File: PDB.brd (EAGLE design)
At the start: 125.9 x 103 mm, 50 parts, among them J1 B06B-HCMKK, J2 B06B-HCMKK, J3 SS-6488-NF-A431, J4 SS-6488-NF-A431, J5 B06B-HCMKK, J6 B03B-HCMKS, J7 B03B-HCMKS, J8 SS-6488-NF-A431

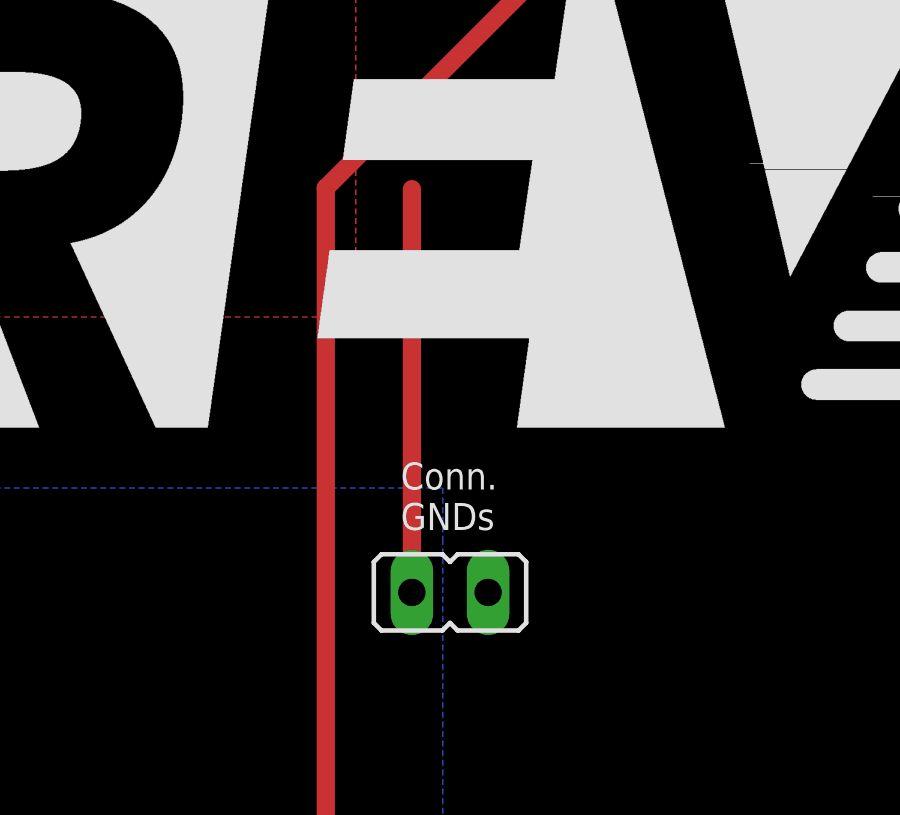
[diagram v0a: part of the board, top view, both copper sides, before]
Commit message: Schematic first version
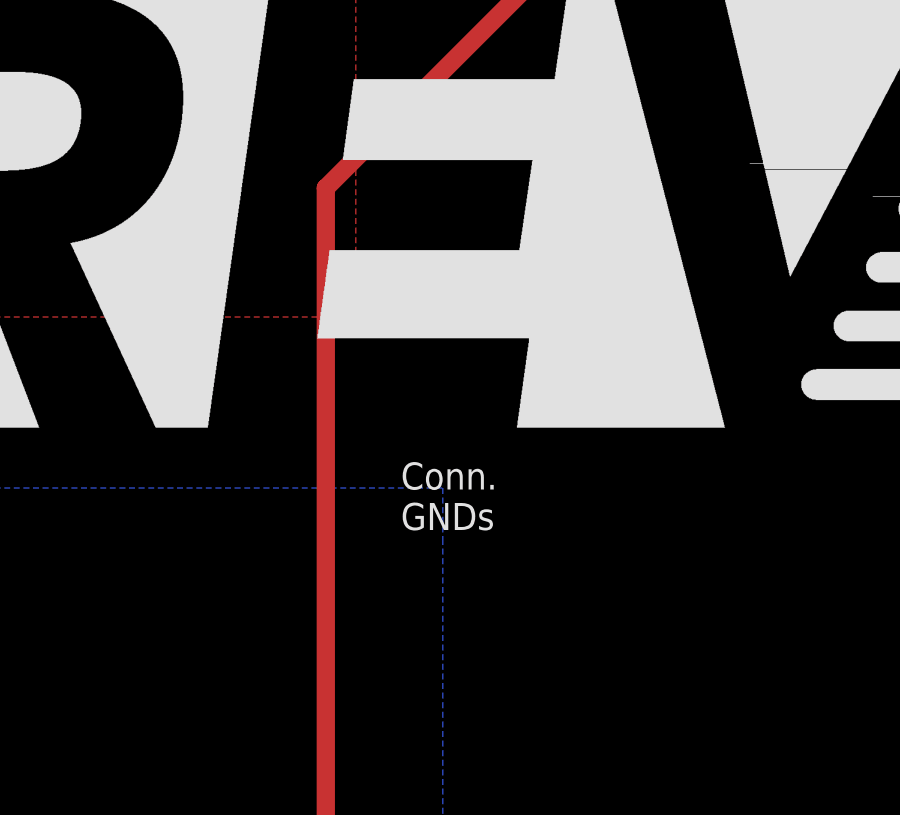
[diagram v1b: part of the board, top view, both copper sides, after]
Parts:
- removed JP1: (no value), jumper:JP1
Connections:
- removed net µC_GND: JP1.2
- new net VIPER: J2.3
- net GND: no longer JP1.1
- net HORN: now also J2.4
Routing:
- net µC_GND: track 13.4 -> 0.00 mm
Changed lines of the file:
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@@
 <element name="TRACO" library="master_library" package="SIP3" value="TRACO-TSR-1-2450" x="120.78" y="101.56" smashed="yes"/>
 <element name="LM2940" library="master_library" package="SOT230P700X180-4" package3d_urn="urn:adsk.eagle:package:8814566/1" value="LM2940LM" x="30.48" y="112.8" smashed="yes"/>
-<element name="JP1" library="jumper" library_urn="urn:adsk.eagle:library:252" package="JP1" package3d_urn="urn:adsk.eagle:package:15455/1" value="" x="105.14" y="66.52" smashed="yes" rot="R90">
-<attribute name="POPULARITY" value="15" x="105.14" y="66.52" size="1.778" layer="27" rot="R90" display="off"/>
-<attribute name="VALUE" x="107.68" y="69.441" size="1.27" layer="27" ratio="10" rot="R180"/>
-</element>
 <element name="C5" library="SparkFun-Capacitors" library_urn="urn:adsk.eagle:library:510" package="PANASONIC_C" package3d_urn="urn:adsk.eagle:package:37430/1" value="47uF" x="22.2" y="112.9" smashed="yes" rot="R270">
 <attribute name="NAME" x="24.867" y="112.9" size="0.6096" layer="25" font="vector" ratio="20" rot="R270" align="bottom-center"/>
@@
 </signal>
 <signal name="µC_GND">
-<contactref element="JP1" pad="2"/>
 <polygon width="0.2" layer="16" isolate="0.254">
 <vertex x="104.9" y="68.3"/>
@@
 <vertex x="104.9" y="70"/>
 </polygon>
-<wire x1="103.87" y1="66.52" x2="103.87" y2="79.962" width="0.6096" layer="1"/>
 </signal>
 <signal name="5V_REG">
@@
 <wire x1="106.34" y1="108.42" x2="103.6645" y2="108.42" width="0.6096" layer="1"/>
 <wire x1="103.435" y1="108.312" x2="103.6645" y2="108.42" width="0.6096" layer="1"/>
-<contactref element="JP1" pad="1"/>
 <contactref element="R5" pad="2"/>
 <contactref element="HAZ_R" pad="2"/>
@@
 <wire x1="16.36" y1="88.56" x2="27.4532" y2="112.8" width="0" layer="19" extent="1-1"/>
 <wire x1="-13.92" y1="89.82" x2="15.72" y2="86.28" width="0" layer="19" extent="1-1"/>
-<wire x1="106.41" y1="66.52" x2="121.35" y2="97.6" width="0" layer="19" extent="1-1"/>
 <wire x1="1.32" y1="54.26" x2="15.72" y2="86.28" width="0" layer="19" extent="1-1"/>
 <wire x1="2.3" y1="20" x2="1.32" y2="54.26" width="0" layer="19" extent="1-1"/>
@@
 <wire x1="-43.83" y1="18.84" x2="-26.73" y2="18.84" width="0" layer="19" extent="1-1"/>
 <wire x1="-31.9" y1="-8.2" x2="-26.73" y2="18.84" width="0" layer="19" extent="1-1"/>
-<wire x1="66.48" y1="67.788" x2="106.41" y2="66.52" width="0" layer="19" extent="1-1"/>
+<wire x1="66.48" y1="67.788" x2="69.2" y2="109" width="0" layer="19" extent="1-1"/>
 <wire x1="-39.52" y1="-76.9" x2="-31.9" y2="-8.2" width="0" layer="19" extent="1-1"/>
 <wire x1="-47.82" y1="-91.11" x2="-39.52" y2="-76.9" width="0" layer="19" extent="1-1"/>
@@
 <signal name="HORN">
 <contactref element="U$5" pad="SWB"/>
+<contactref element="J2" pad="4"/>
+<wire x1="-2.78" y1="5.9" x2="-32.58" y2="-91.11" width="0" layer="19" extent="1-1"/>
 </signal>
 <signal name="MOSI_SW">
@@
 <wire x1="-13.92" y1="72.04" x2="-54.58" y2="-85.3" width="0" layer="19" extent="1-1"/>
 </signal>
+<signal name="VIPER">
+<contactref element="J2" pad="3"/>
+</signal>
 </signals>

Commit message: Board layout proposal
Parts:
- moved J8 207.7 mm to (112.5, 27.1), turned to 90 degrees
- moved U$6 198.5 mm to (27.0, 89.2), turned to 270 degrees
- moved U$5 194.8 mm to (42.8, 88.9), turned to 270 degrees
- moved HORN 174.8 mm to (72.3, 80.0)
- moved J2 161.9 mm to (78.0, 141.5)
- moved J5 150.4 mm to (92.1, 54.4), flipped to the bottom
- moved POWER1 145.3 mm to (58.6, 62.9)
- moved J1 135.2 mm to (48.3, 141.8)
- moved J6 134.1 mm to (22.4, 52.2), turned to 90 degrees
- moved R1 133.6 mm to (52.8, 62.8), turned to 180 degrees
- moved U$4 129.0 mm to (64.0, 54.6), turned to 90 degrees
- moved J4 127.6 mm to (82.2, 7.00)
- moved J7 123.9 mm to (22.7, 27.1), turned to 90 degrees
- moved U$2 111.0 mm to (44.8, 53.9), turned to 270 degrees
- moved J3 78.4 mm to (49.8, 6.50)
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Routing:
- net BRAKE_SNS: track 85.4 -> 17.8 mm, vias 1 -> 0
- net BRAKE_SIG: track 50.3 -> 0.00 mm
- net HAZ_L_SIG: track 46.5 -> 0.12 mm, vias 1 -> 0
- net 5V_REG: track 33.0 -> 3.99 mm
- net HAZ_R_SIG: track 33.9 -> 8.31 mm
- net H7: track 6.44 -> 32.0 mm
- net REARLIGHT_SIG: track 10.9 -> 0.00 mm
- net H4: track 8.35 -> 0.00 mm
- net HEADLIGHT_SIG: track 7.43 -> 0.00 mm
- net H3: track 6.53 -> 11.7 mm
- net H2: track 7.72 -> 11.1 mm
- net H8: track 6.54 -> 7.95 mm
- net CLK: track 0.82 -> 0.00 mm
- removed copper zone on layer 1, net 12V_IN
- removed copper zone on layer 16, net µC_GND
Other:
- board size 125.9 x 103 mm -> 126.8 x 162.5 mm
- board text removed: "12V IN"
- board text removed: "22uF"
- board text removed: "4.7k"
- board text removed: "555"
- board text removed: "ADD 1"
- board text removed: "Add 1"
- board text removed: "Add 2"
- board text removed: "BRAKE"
- board text removed: "Brake Light"
- board text removed: "Brake Sensor"
- board text removed: "Conn. GNDs"
- board text removed: "HL"
- board text removed: "Head Lights"
- board text removed: "ON"
- board text removed: "RL"
- board text removed: "Rear Lights"
- board text removed: "TURN_L"
- board text removed: "TURN_R"
- board text removed: "Wiper"
- board text removed: "µC"
- board text removed: "µC GND"

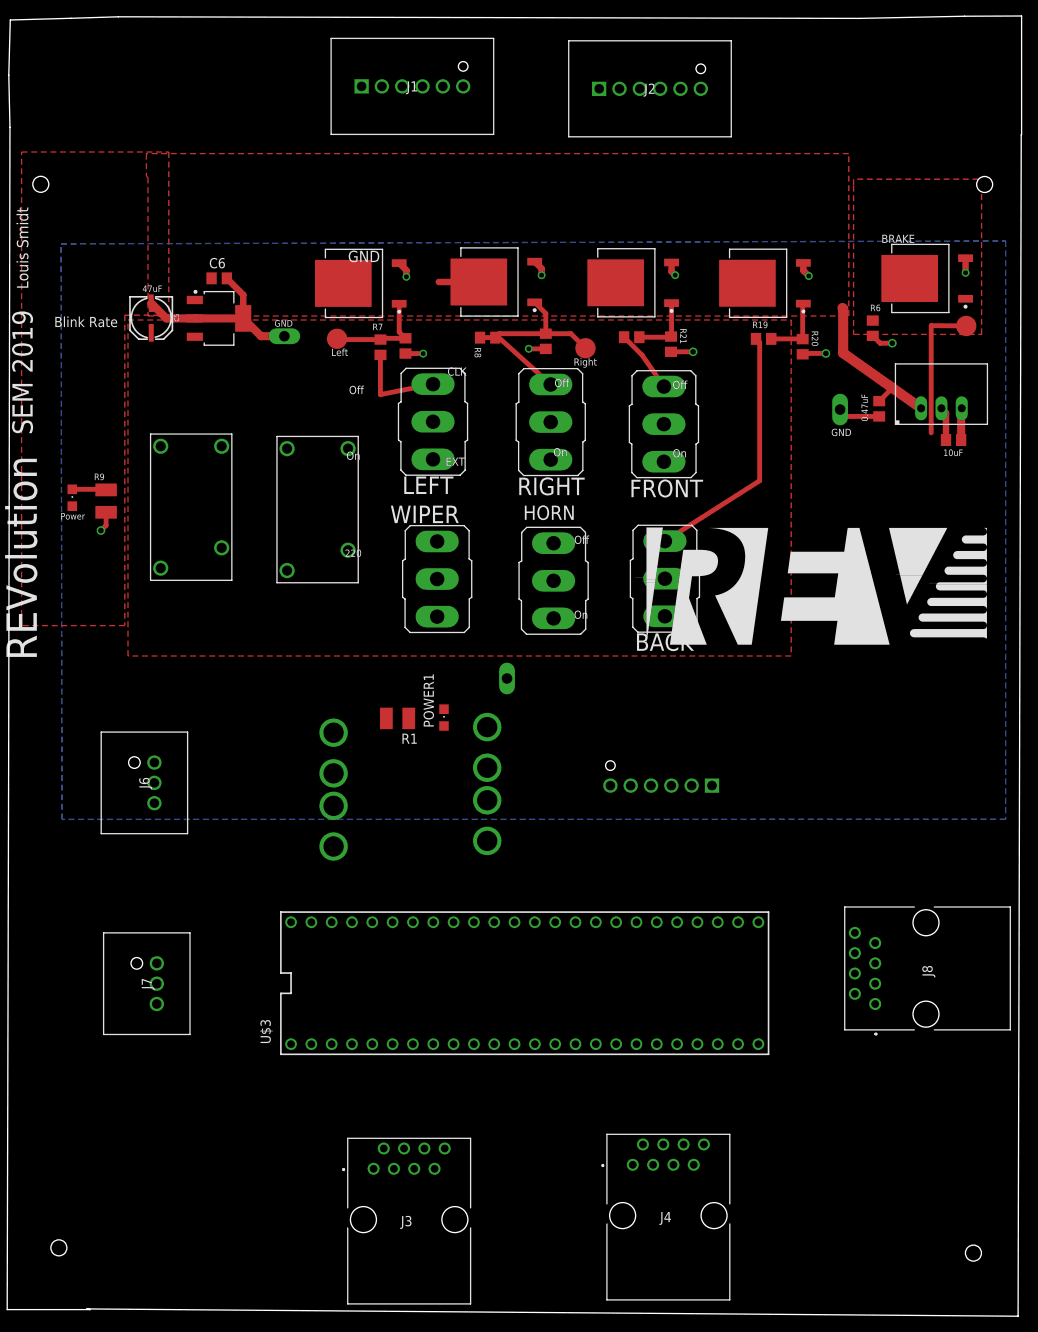
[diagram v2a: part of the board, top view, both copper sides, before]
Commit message: Board first version
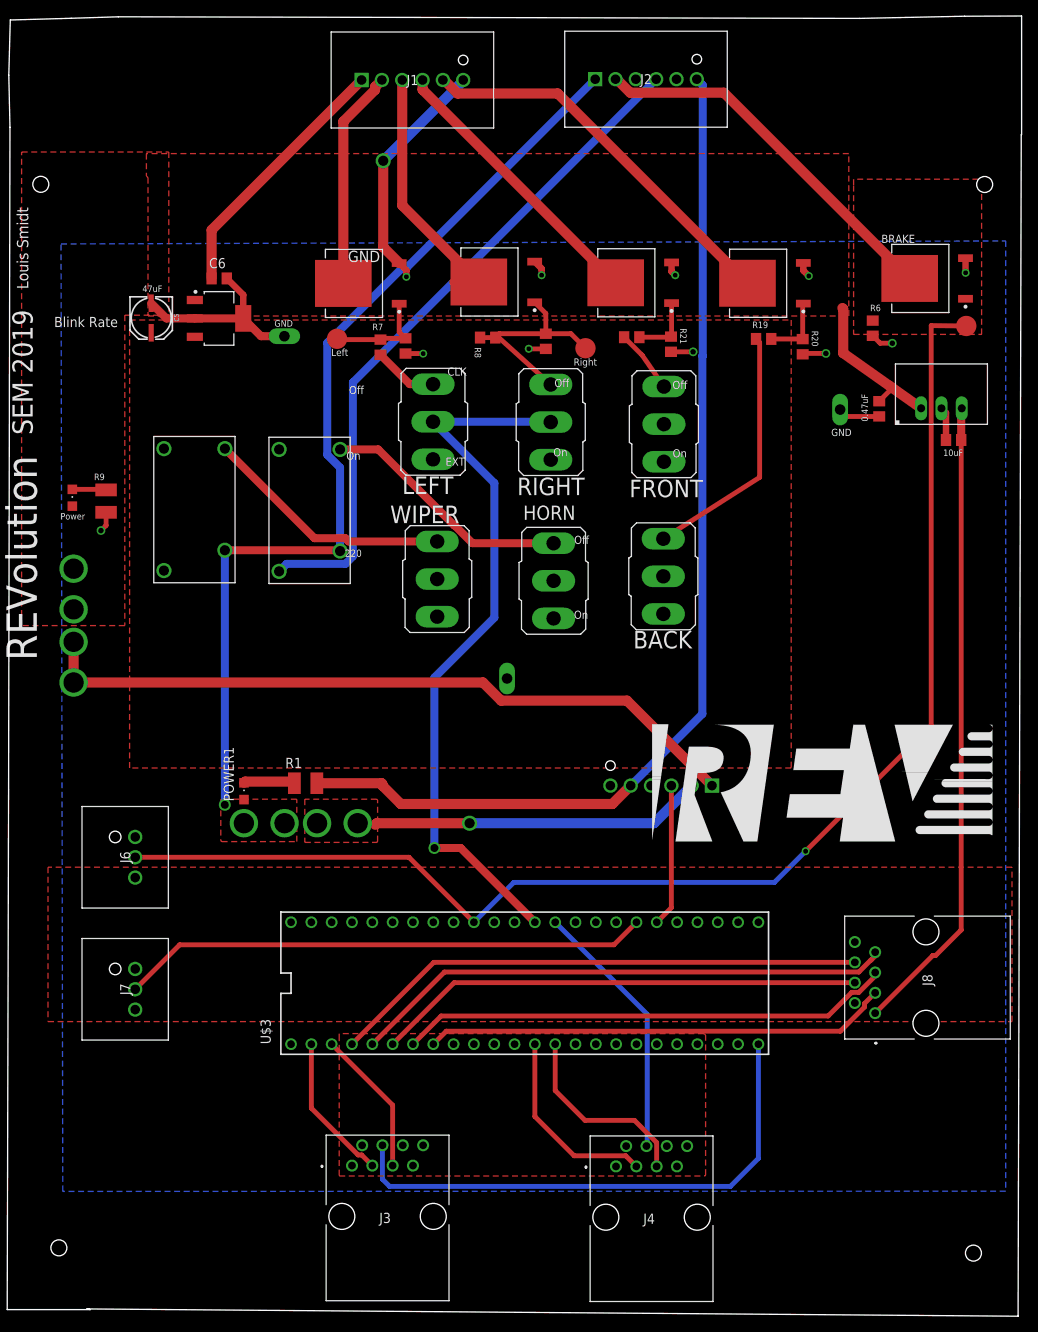
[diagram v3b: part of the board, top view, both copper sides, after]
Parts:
- moved U$2 38.4 mm to (12.3, 74.4)
- moved POWER1 26.6 mm to (33.6, 53.7)
- moved U$4 23.8 mm to (40.7, 49.7), turned to 180 degrees
- moved R1 14.1 mm to (41.3, 54.7), turned to 0 degrees
- moved J6 9.60 mm to (20.0, 42.9)
- moved J7 2.79 mm to (20.0, 26.4)
- moved J3 2.73 mm to (47.1, 6.90)
- moved J4 2.11 mm to (80.1, 6.80)
- moved J2 1.30 mm to (77.5, 142.7)
- moved J8 1.14 mm to (112.5, 26.0)
- moved U$5 1.00 mm to (41.8, 88.8)
- moved J1 0.80 mm to (48.3, 142.6)
- moved U$6 0.50 mm to (27.4, 88.9)
- moved BACK 0.36 mm to (86.0, 80.6)
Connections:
- removed net 5V: J7.1
- net 5V_REG: now also J7.1
- net CLK_SW: now also J8.6; no longer J8.4
- net CS: now also J8.4; no longer J8.6
- net MOSI_SW: now also J8.7; no longer J8.3
- net RESET: now also J8.3; no longer J8.7
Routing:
- net BRAKE_SNS: track 17.8 -> 167.4 mm, vias 0 -> 1
- net IGND: track 0.00 -> 133.7 mm
- net IVDD: track 0.00 -> 120.2 mm, vias 0 -> 1
- net CLK: track 0.00 -> 90.7 mm, vias 0 -> 1
- net N$7: track 0.00 -> 90.2 mm
- net HORN: track 0.00 -> 85.3 mm
- net 5V_REG: track 3.99 -> 80.3 mm
- net MOSI_SW: track 0.00 -> 67.9 mm
- net CLK_A: track 0.00 -> 67.3 mm
- net CLK_SW: track 0.00 -> 67.1 mm
- net PEDAL_SNS: track 0.00 -> 66.1 mm
- net DC: track 0.00 -> 61.7 mm
- net CS: track 0.00 -> 61.0 mm
- net RESET: track 0.00 -> 58.2 mm
- net REARLIGHT_SIG: track 0.00 -> 48.6 mm
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- added copper zone on layer 1, net 3.3V
- added copper zone on layer 1, net 5V_REG
- added copper zone on layer 1, net IVDD
- added copper zone on layer 1, net N$8
